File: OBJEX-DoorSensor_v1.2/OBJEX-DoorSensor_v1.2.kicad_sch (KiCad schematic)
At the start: 3 parts

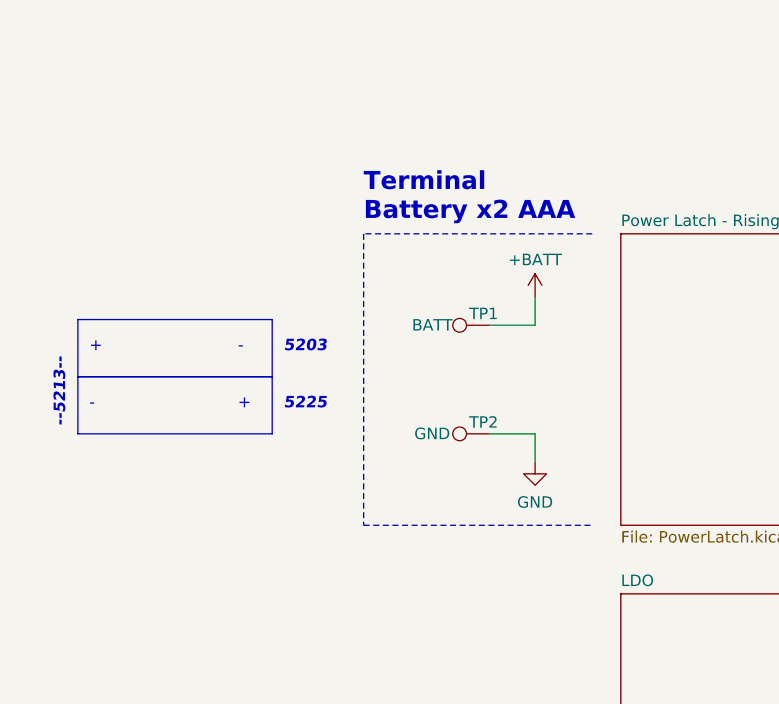
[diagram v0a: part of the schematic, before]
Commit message: update
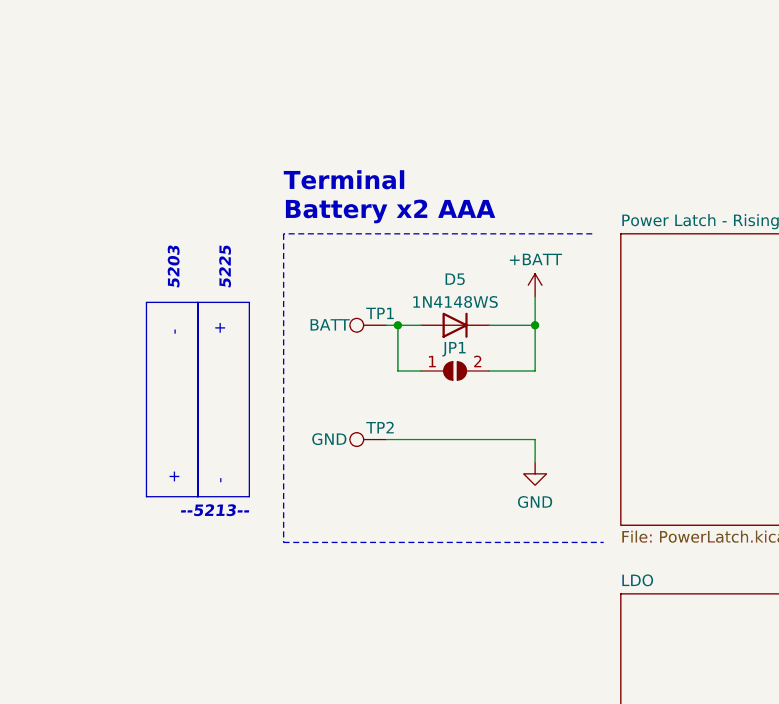
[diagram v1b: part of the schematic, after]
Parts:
- added D5: 1N4148WS, Diode_SMD:D_SOD-323, symbol Diode:1N4148WS
- added JP1: SolderJumper_2_Open, Jumper:SolderJumper-2_P1.3mm_Open_RoundedPad1.0x1.5mm, symbol Jumper:SolderJumper_2_Open
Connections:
- net +BATT: now also D5.1 (K), JP1.2 (B); no longer TP1.1
- new net: D5.2 (A), JP1.1 (A), TP1.1
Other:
- moved on the sheet: TP1, TP2
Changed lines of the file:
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@@
     (comment 2 "Designer: Salvatore Raccardi")
+  )
+  (junction (at 71.12 72.39) (diameter 0) (color 0 0 0 0)
+  )
+  (junction (at 55.88 72.39) (diameter 0) (color 0 0 0 0)
   )
   (no_connect (at 200.66 118.745))
   (no_connect (at 170.18 116.205))
+  (wire (pts (xy 66.04 77.47) (xy 71.12 77.47))
+    (stroke (width 0) (type default))
+  )
   (wire (pts (xy 138.43 79.375) (xy 156.21 79.375))
     (stroke (width 0) (type default))
@@
     (stroke (width 0) (type default))
   )
-  (polyline (pts (xy 52.07 62.23) (xy 52.07 94.615))
+  (polyline (pts (xy 43.18 62.23) (xy 43.18 96.52))
     (stroke (width 0) (type dash_dot))
   )
-  (polyline (pts (xy 52.07 94.615) (xy 77.47 94.615))
+  (wire (pts (xy 71.12 69.215) (xy 71.12 72.39))
+    (stroke (width 0) (type default))
+  )
+  (wire (pts (xy 217.17 116.205) (xy 217.17 89.535))
+    (stroke (width 0) (type default))
+  )
+  (wire (pts (xy 71.12 77.47) (xy 71.12 72.39))
+    (stroke (width 0) (type default))
+  )
+  (wire (pts (xy 170.18 118.745) (xy 168.148 118.745))
+    (stroke (width 0) (type default))
+  )
+  (wire (pts (xy 55.88 77.47) (xy 58.42 77.47))
+    (stroke (width 0) (type default))
+  )
+  (polyline (pts (xy 43.18 96.52) (xy 78.74 96.52))
     (stroke (width 0) (type dash_dot))
   )
-  (wire (pts (xy 71.12 69.215) (xy 71.12 72.39))
-    (stroke (width 0) (type default))
-  )
-  (wire (pts (xy 217.17 116.205) (xy 217.17 89.535))
-    (stroke (width 0) (type default))
-  )
-  (wire (pts (xy 170.18 118.745) (xy 168.148 118.745))
-    (stroke (width 0) (type default))
-  )
-  (wire (pts (xy 71.12 84.455) (xy 71.12 87.63))
+  (wire (pts (xy 71.12 85.09) (xy 71.12 87.63))
     (stroke (width 0) (type default))
   )
@@
     (stroke (width 0) (type default))
   )
-  (wire (pts (xy 66.04 84.455) (xy 71.12 84.455))
+  (wire (pts (xy 54.61 85.09) (xy 71.12 85.09))
     (stroke (width 0) (type default))
   )
@@
     (stroke (width 0) (type default))
   )
-  (polyline (pts (xy 77.47 62.23) (xy 52.07 62.23))
+  (polyline (pts (xy 77.47 62.23) (xy 43.18 62.23))
     (stroke (width 0) (type dash_dot))
   )
+  (wire (pts (xy 55.88 72.39) (xy 55.88 77.47))
+    (stroke (width 0) (type default))
+  )
+  (wire (pts (xy 55.88 72.39) (xy 58.42 72.39))
+    (stroke (width 0) (type default))
+  )
+  (wire (pts (xy 54.61 72.39) (xy 55.88 72.39))
+    (stroke (width 0) (type default))
+  )
   (wire (pts (xy 138.43 74.295) (xy 156.21 74.295))
     (stroke (width 0) (type default))
   )
-  (rectangle (start 20.32 78.105) (end 41.91 84.455)
+  (rectangle (start 27.94 69.85) (end 33.655 91.44)
     (stroke (width 0) (type default))
     (fill (type none))
@@
     (fill (type none))
   )
-  (rectangle (start 20.32 71.755) (end 41.91 78.105)
+  (rectangle (start 33.655 69.85) (end 39.37 91.44)
     (stroke (width 0) (type default))
     (fill (type none))
@@
     (effects (font (size 1.2 1.2)) (justify left bottom))
   )
-  (text "5225" (at 43.18 81.915 0)
+  (text "5225" (at 37.465 68.58 90)
     (effects (font (size 1.27 1.27) bold italic) (justify left bottom))
   )
-  (text "+" (at 38.1 81.915 0)
+  (text "+" (at 36.83 73.66 90)
     (effects (font (size 1.27 1.27)) (justify left bottom))
   )
-  (text "-\n" (at 38.1 75.565 0)
+  (text "-\n" (at 31.75 73.66 90)
     (effects (font (size 1.27 1.27)) (justify left bottom))
   )
-  (text "Terminal\nBattery x2 AAA" (at 52.07 60.96 0)
+  (text "Terminal\nBattery x2 AAA" (at 43.18 60.96 0)
     (effects (font (size 2 2) (thickness 0.254) bold) (justify left bottom))
   )
@@
     (effects (font (size 4 4) (thickness 0.6) bold) (justify left bottom))
   )
-  (text "+" (at 21.59 75.565 0)
+  (text "+" (at 31.75 90.17 90)
     (effects (font (size 1.27 1.27)) (justify left bottom))
   )
-  (text "--5213--\n" (at 19.05 83.82 90)
-    (effects (font (size 1.27 1.27) (thickness 0.254) bold italic) (justify left bottom))
-  )
-  (text "-\n" (at 21.59 81.915 0)
+  (text "--5213--\n" (at 39.37 93.98 0)
+    (effects (font (size 1.27 1.27) (thickness 0.254) bold italic) (justify right bottom))
+  )
+  (text "-\n" (at 36.83 90.17 90)
     (effects (font (size 1.27 1.27)) (justify left bottom))
   )
-  (text "5203\n" (at 43.18 75.565 0)
+  (text "5203\n" (at 31.75 68.58 90)
     (effects (font (size 1.27 1.27) (thickness 0.254) bold italic) (justify left bottom))
   )
@@
     )
   )
-  (symbol (lib_id "Connector:TestPoint") (at 66.04 84.455 90) (unit 1)
+  (symbol (lib_id "Connector:TestPoint") (at 54.61 85.09 90) (unit 1)
     (in_bom yes) (on_board yes) (dnp no)
-    (property "Reference" "TP2" (at 65.405 83.185 90)
-      (effects (font (size 1.27 1.27)))
-    )
-    (property "Value" "GND" (at 59.69 84.455 90)
-      (effects (font (size 1.27 1.27)))
-    )
-    (property "Footprint" "TestPoint:TestPoint_Pad_1.5x1.5mm" (at 66.04 79.375 0)
-      (effects (font (size 1.27 1.27)) hide)
-    )
-    (property "Datasheet" "~" (at 66.04 79.375 0)
+    (property "Reference" "TP2" (at 53.975 83.82 90)
+      (effects (font (size 1.27 1.27)))
+    )
+    (property "Value" "GND" (at 48.26 85.09 90)
+      (effects (font (size 1.27 1.27)))
+    )
+    (property "Footprint" "TestPoint:TestPoint_Pad_1.5x1.5mm" (at 54.61 80.01 0)
+      (effects (font (size 1.27 1.27)) hide)
+    )
+    (property "Datasheet" "~" (at 54.61 80.01 0)
       (effects (font (size 1.27 1.27)) hide)
     )
@@
     )
   )
+  (symbol (lib_id "Diode:1N4148WS") (at 62.23 72.39 180) (unit 1)
+    (in_bom yes) (on_board yes) (dnp no) (fields_autoplaced)
+    (property "Reference" "D5" (at 62.23 67.31 0)
+      (effects (font (size 1.27 1.27)))
+    )
+    (property "Value" "1N4148WS" (at 62.23 69.85 0)
+      (effects (font (size 1.27 1.27)))
+    )
+    (property "Footprint" "Diode_SMD:D_SOD-323" (at 62.23 67.945 0)
+      (effects (font (size 1.27 1.27)) hide)
+    )
+    (property "Datasheet" "https://www.vishay.com/docs/85751/1n4148ws.pdf" (at 62.23 72.39 0)
+      (effects (font (size 1.27 1.27)) hide)
+    )
+    (property "Sim.Device" "D" (at 62.23 72.39 0)
+      (effects (font (size 1.27 1.27)) hide)
+    )
+    (property "Sim.Pins" "1=K 2=A" (at 62.23 72.39 0)
+      (effects (font (size 1.27 1.27)) hide)
+    )
+    (pin "1")
+    (pin "2")
+    (instances
+      (project "OBJEX-DoorSensor_v1.2"
+        (path "/dfd7f005-123d-49c6-a596-950b92e8aba7/49ed0aa1-c89e-4756-9039-f42ff518440c"
+          (reference "D5") (unit 1)
+        )
+        (path "/dfd7f005-123d-49c6-a596-950b92e8aba7"
+          (reference "D5") (unit 1)
+        )
+      )
+    )
+  )
+  (symbol (lib_id "Jumper:SolderJumper_2_Open") (at 62.23 77.47 0) (unit 1)
+    (in_bom yes) (on_board yes) (dnp no) (fields_autoplaced)
+    (property "Reference" "JP1" (at 62.23 74.93 0)
+      (effects (font (size 1.27 1.27)))
+    )
+    (property "Value" "SolderJumper_2_Open" (at 62.23 74.93 0)
+      (effects (font (size 1.27 1.27)) hide)
+    )
+    (property "Footprint" "Jumper:SolderJumper-2_P1.3mm_Open_RoundedPad1.0x1.5mm" (at 62.23 77.47 0)
+      (effects (font (size 1.27 1.27)) hide)
+    )
+    (property "Datasheet" "~" (at 62.23 77.47 0)
+      (effects (font (size 1.27 1.27)) hide)
+    )
+    (pin "1")
+    (pin "2")
+    (instances
+      (project "OBJEX-DoorSensor_v1.2"
+        (path "/dfd7f005-123d-49c6-a596-950b92e8aba7"
+          (reference "JP1") (unit 1)
+        )
+      )
+    )
+  )
   (symbol (lib_id "power:GND") (at 168.148 122.8852 0) (unit 1)
     (in_bom yes) (on_board yes) (dnp no)
@@
     )
   )
-  (symbol (lib_id "Connector:TestPoint") (at 66.04 72.39 90) (unit 1)
+  (symbol (lib_id "Connector:TestPoint") (at 54.61 72.39 90) (unit 1)
     (in_bom yes) (on_board yes) (dnp no)
-    (property "Reference" "TP1" (at 65.405 71.12 90)
-      (effects (font (size 1.27 1.27)))
-    )
-    (property "Value" "BATT" (at 59.69 72.39 90)
-      (effects (font (size 1.27 1.27)))
-    )
-    (property "Footprint" "TestPoint:TestPoint_Pad_1.5x1.5mm" (at 66.04 67.31 0)
-      (effects (font (size 1.27 1.27)) hide)
-    )
-    (property "Datasheet" "~" (at 66.04 67.31 0)
-      (effects (font (size 1.27 1.27)) hide)
-    )
+    (property "Reference" "TP1" (at 53.975 71.12 90)
+      (effects (font (size 1.27 1.27)))
+    )
+    (property "Value" "BATT" (at 48.26 72.39 90)
+      (effects (font (size 1.27 1.27)))
+    )
+    (property "Footprint" "TestPoint:TestPoint_Pad_1.5x1.5mm" (at 54.61 67.31 0)
+      (effects (font (size 1.27 1.27)) hide)
+    )
+    (property "Datasheet" "~" (at 54.61 67.31 0)
+      (effects (font (size 1.27 1.27)) hide)
+    )

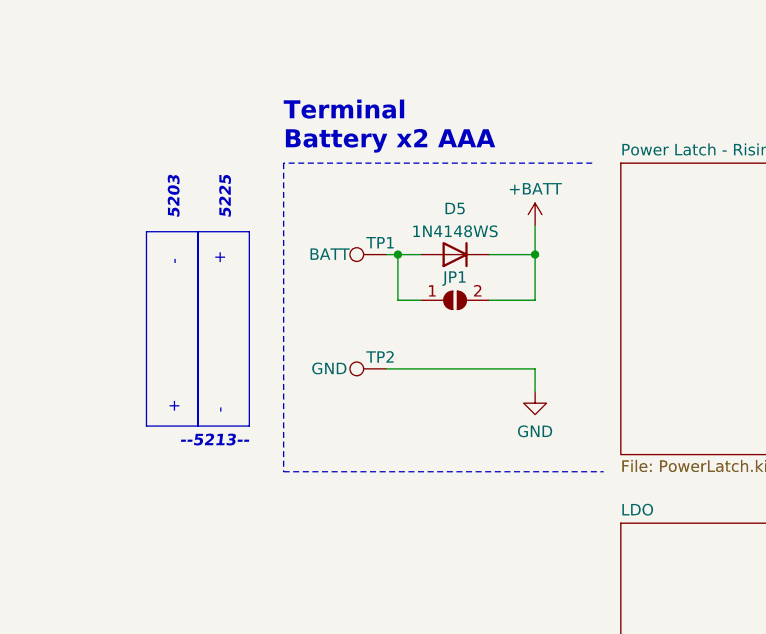
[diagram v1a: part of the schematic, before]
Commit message: Start PCB design
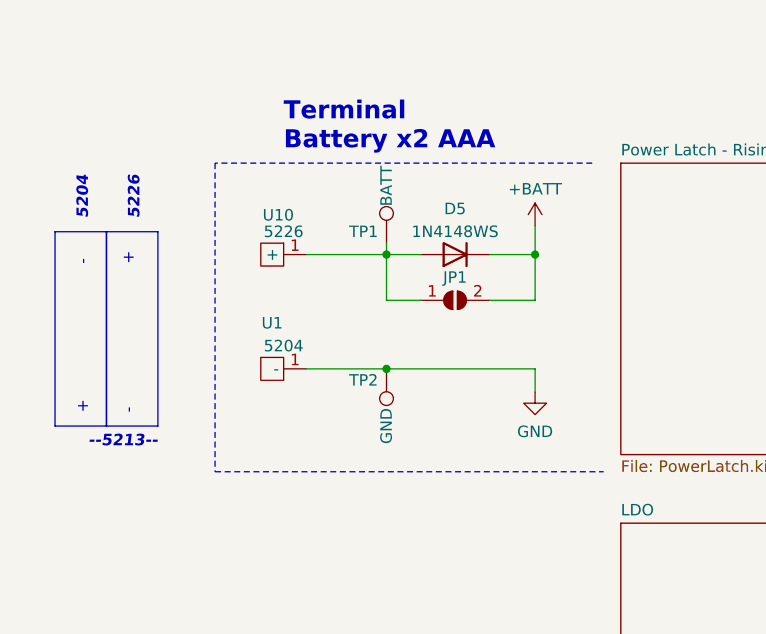
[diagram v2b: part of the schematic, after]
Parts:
- added U1: 5204, BatteryTerminal:5204, symbol BatteryTerminal:5204
- added U10: 5226, BatteryTerminal:5226, symbol BatteryTerminal:5226
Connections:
- net GND: now also U1.1 (-)
- net at D5.2 (A), JP1.1 (A), TP1.1: now also U10.1 (+)
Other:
- note added: "5204"
- note added: "5226"
- note removed: "5203"
- note removed: "5225"
- moved on the sheet: TP1, TP2
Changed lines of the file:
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@@
     (comment 2 "Designer: Salvatore Raccardi")
   )
+  (junction (at 54.61 85.09) (diameter 0) (color 0 0 0 0)
+  )
+  (junction (at 54.61 72.39) (diameter 0) (color 0 0 0 0)
+  )
   (junction (at 71.12 72.39) (diameter 0) (color 0 0 0 0)
-  )
-  (junction (at 55.88 72.39) (diameter 0) (color 0 0 0 0)
   )
   (no_connect (at 200.66 118.745))
@@
     (stroke (width 0) (type default))
   )
-  (polyline (pts (xy 43.18 62.23) (xy 43.18 96.52))
+  (wire (pts (xy 45.72 85.09) (xy 54.61 85.09))
+    (stroke (width 0) (type default))
+  )
+  (polyline (pts (xy 35.56 62.23) (xy 35.56 96.52))
     (stroke (width 0) (type dash_dot))
   )
@@
     (stroke (width 0) (type default))
   )
-  (wire (pts (xy 55.88 77.47) (xy 58.42 77.47))
-    (stroke (width 0) (type default))
-  )
-  (polyline (pts (xy 43.18 96.52) (xy 78.74 96.52))
+  (wire (pts (xy 54.61 77.47) (xy 58.42 77.47))
+    (stroke (width 0) (type default))
+  )
+  (polyline (pts (xy 35.56 96.52) (xy 78.74 96.52))
     (stroke (width 0) (type dash_dot))
   )
+  (wire (pts (xy 45.72 72.39) (xy 54.61 72.39))
+    (stroke (width 0) (type default))
+  )
+  (wire (pts (xy 54.61 71.12) (xy 54.61 72.39))
+    (stroke (width 0) (type default))
+  )
   (wire (pts (xy 71.12 85.09) (xy 71.12 87.63))
     (stroke (width 0) (type default))
@@
     (stroke (width 0) (type default))
   )
-  (polyline (pts (xy 77.47 62.23) (xy 43.18 62.23))
+  (polyline (pts (xy 77.47 62.23) (xy 35.56 62.23))
     (stroke (width 0) (type dash_dot))
   )
-  (wire (pts (xy 55.88 72.39) (xy 55.88 77.47))
-    (stroke (width 0) (type default))
-  )
-  (wire (pts (xy 55.88 72.39) (xy 58.42 72.39))
-    (stroke (width 0) (type default))
-  )
-  (wire (pts (xy 54.61 72.39) (xy 55.88 72.39))
+  (wire (pts (xy 54.61 72.39) (xy 58.42 72.39))
+    (stroke (width 0) (type default))
+  )
+  (wire (pts (xy 54.61 77.47) (xy 54.61 72.39))
     (stroke (width 0) (type default))
   )
@@
     (stroke (width 0) (type default))
   )
-  (rectangle (start 27.94 69.85) (end 33.655 91.44)
+  (rectangle (start 17.78 69.85) (end 23.495 91.44)
     (stroke (width 0) (type default))
     (fill (type none))
@@
     (fill (type none))
   )
-  (rectangle (start 33.655 69.85) (end 39.37 91.44)
+  (rectangle (start 23.495 69.85) (end 29.21 91.44)
     (stroke (width 0) (type default))
     (fill (type none))
@@
     (effects (font (size 1.2 1.2)) (justify left bottom))
   )
-  (text "5225" (at 37.465 68.58 90)
+  (text "5226\n" (at 27.305 68.58 90)
     (effects (font (size 1.27 1.27) bold italic) (justify left bottom))
   )
-  (text "+" (at 36.83 73.66 90)
+  (text "+" (at 26.67 73.66 90)
     (effects (font (size 1.27 1.27)) (justify left bottom))
   )
-  (text "-\n" (at 31.75 73.66 90)
+  (text "-\n" (at 21.59 73.66 90)
     (effects (font (size 1.27 1.27)) (justify left bottom))
   )
@@
     (effects (font (size 4 4) (thickness 0.6) bold) (justify left bottom))
   )
-  (text "+" (at 31.75 90.17 90)
+  (text "+" (at 21.59 90.17 90)
     (effects (font (size 1.27 1.27)) (justify left bottom))
   )
-  (text "--5213--\n" (at 39.37 93.98 0)
+  (text "--5213--\n" (at 29.21 93.98 0)
     (effects (font (size 1.27 1.27) (thickness 0.254) bold italic) (justify right bottom))
   )
-  (text "-\n" (at 36.83 90.17 90)
+  (text "-\n" (at 26.67 90.17 90)
     (effects (font (size 1.27 1.27)) (justify left bottom))
   )
-  (text "5203\n" (at 31.75 68.58 90)
+  (text "5204\n" (at 21.59 68.58 90)
     (effects (font (size 1.27 1.27) (thickness 0.254) bold italic) (justify left bottom))
   )
@@
     )
   )
-  (symbol (lib_id "Connector:TestPoint") (at 54.61 85.09 90) (unit 1)
+  (symbol (lib_id "Connector:TestPoint") (at 54.61 85.09 180) (unit 1)
     (in_bom yes) (on_board yes) (dnp no)
-    (property "Reference" "TP2" (at 53.975 83.82 90)
-      (effects (font (size 1.27 1.27)))
-    )
-    (property "Value" "GND" (at 48.26 85.09 90)
-      (effects (font (size 1.27 1.27)))
-    )
-    (property "Footprint" "TestPoint:TestPoint_Pad_1.5x1.5mm" (at 54.61 80.01 0)
-      (effects (font (size 1.27 1.27)) hide)
-    )
-    (property "Datasheet" "~" (at 54.61 80.01 0)
+    (property "Reference" "TP2" (at 52.07 86.36 0)
+      (effects (font (size 1.27 1.27)))
+    )
+    (property "Value" "GND" (at 54.61 91.44 90)
+      (effects (font (size 1.27 1.27)))
+    )
+    (property "Footprint" "TestPoint:TestPoint_Pad_1.5x1.5mm" (at 49.53 85.09 0)
+      (effects (font (size 1.27 1.27)) hide)
+    )
+    (property "Datasheet" "~" (at 49.53 85.09 0)
       (effects (font (size 1.27 1.27)) hide)
     )
@@
         (path "/dfd7f005-123d-49c6-a596-950b92e8aba7"
           (reference "TP2") (unit 1)
+        )
+      )
+    )
+  )
+  (symbol (lib_name "5226_1") (lib_id "BatteryTerminal:5226") (at 43.18 68.58 0) (unit 1)
+    (in_bom yes) (on_board yes) (dnp no)
+    (property "Reference" "U10" (at 42.5876 68.0136 0)
+      (effects (font (size 1.27 1.27)))
+    )
+    (property "Value" "5226" (at 43.18 69.85 0)
+      (effects (font (size 1.27 1.27)))
+    )
+    (property "Footprint" "BatteryTerminal:5226" (at 43.18 68.58 0)
+      (effects (font (size 1.27 1.27)) hide)
+    )
+    (property "Datasheet" "" (at 43.18 68.58 0)
+      (effects (font (size 1.27 1.27)) hide)
+    )
+    (pin "1")
+    (instances
+      (project "OBJEX-DoorSensor_v1.2"
+        (path "/dfd7f005-123d-49c6-a596-950b92e8aba7"
+          (reference "U10") (unit 1)
         )
       )
@@
     )
   )
+  (symbol (lib_id "BatteryTerminal:5204") (at 43.18 81.28 0) (unit 1)
+    (in_bom yes) (on_board yes) (dnp no)
+    (property "Reference" "U1" (at 41.91 80.01 0)
+      (effects (font (size 1.27 1.27)))
+    )
+    (property "Value" "5204" (at 43.18 82.55 0)
+      (effects (font (size 1.27 1.27)))
+    )
+    (property "Footprint" "BatteryTerminal:5204" (at 43.18 81.28 0)
+      (effects (font (size 1.27 1.27)) hide)
+    )
+    (property "Datasheet" "" (at 43.18 81.28 0)
+      (effects (font (size 1.27 1.27)) hide)
+    )
+    (pin "1")
+    (instances
+      (project "OBJEX-DoorSensor_v1.2"
+        (path "/dfd7f005-123d-49c6-a596-950b92e8aba7"
+          (reference "U1") (unit 1)
+        )
+      )
+    )
+  )
   (symbol (lib_id "power:GND") (at 168.148 122.8852 0) (unit 1)
     (in_bom yes) (on_board yes) (dnp no)
@@
     )
   )
-  (symbol (lib_id "Connector:TestPoint") (at 54.61 72.39 90) (unit 1)
+  (symbol (lib_id "Connector:TestPoint") (at 54.61 71.12 0) (unit 1)
     (in_bom yes) (on_board yes) (dnp no)
-    (property "Reference" "TP1" (at 53.975 71.12 90)
-      (effects (font (size 1.27 1.27)))
-    )
-    (property "Value" "BATT" (at 48.26 72.39 90)
-      (effects (font (size 1.27 1.27)))
-    )
-    (property "Footprint" "TestPoint:TestPoint_Pad_1.5x1.5mm" (at 54.61 67.31 0)
-      (effects (font (size 1.27 1.27)) hide)
-    )
-    (property "Datasheet" "~" (at 54.61 67.31 0)
-      (effects (font (size 1.27 1.27)) hide)
-    )
+    (property "Reference" "TP1" (at 52.07 69.85 0)
+      (effects (font (size 1.27 1.27)))
+    )
+    (property "Value" "BATT" (at 54.61 64.77 90)
+      (effects (font (size 1.27 1.27)))
+    )
+    (property "Footprint" "TestPoint:TestPoint_Pad_1.5x1.5mm" (at 59.69 71.12 0)
+      (effects (font (size 1.27 1.27)) hide)
+    )
+    (property "Datasheet" "~" (at 59.69 71.12 0)
+      (effects (font (size 1.27 1.27)) hide)
+    )
